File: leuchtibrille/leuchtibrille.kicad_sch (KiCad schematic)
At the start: 27 parts, among them J1 Conn_01x06_Male, J2 Conn_01x02_Female, J3 USB_C_Receptacle_USB2.0, J4 USB_C_Receptacle_USB2.0, J5 USB_C_Receptacle_USB2.0, SW1 SW_Push, U1 MT3420C, U2 MT3420C, U3 ESP32-WROOM-32

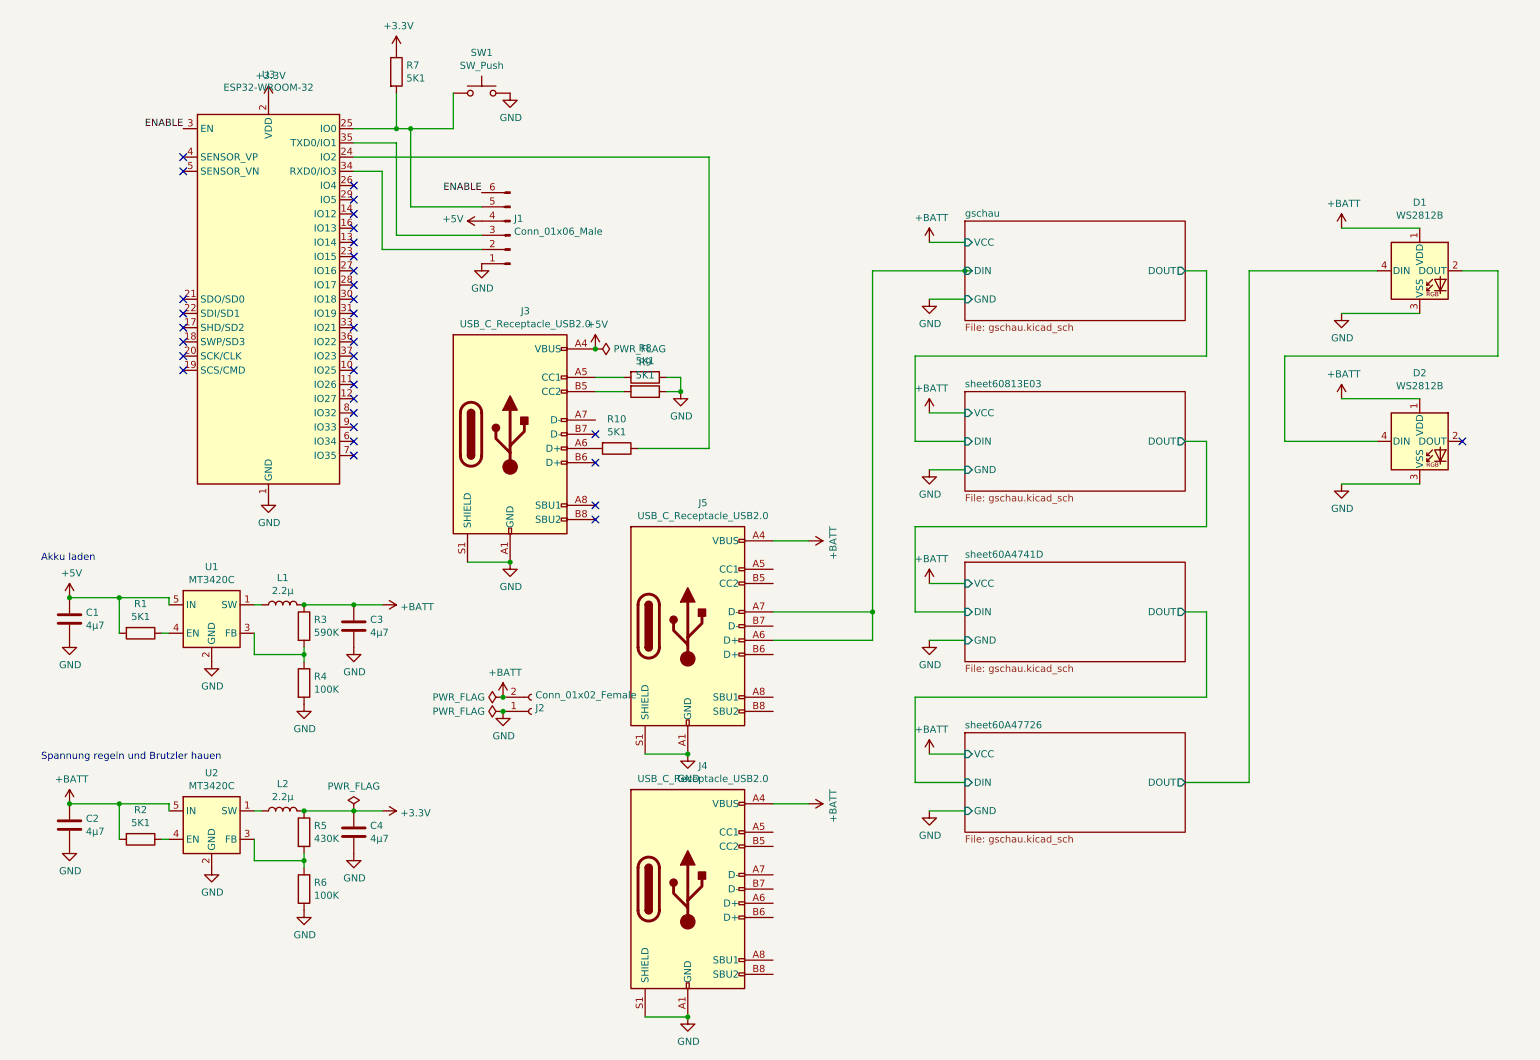
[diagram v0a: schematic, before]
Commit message: Upload of working version
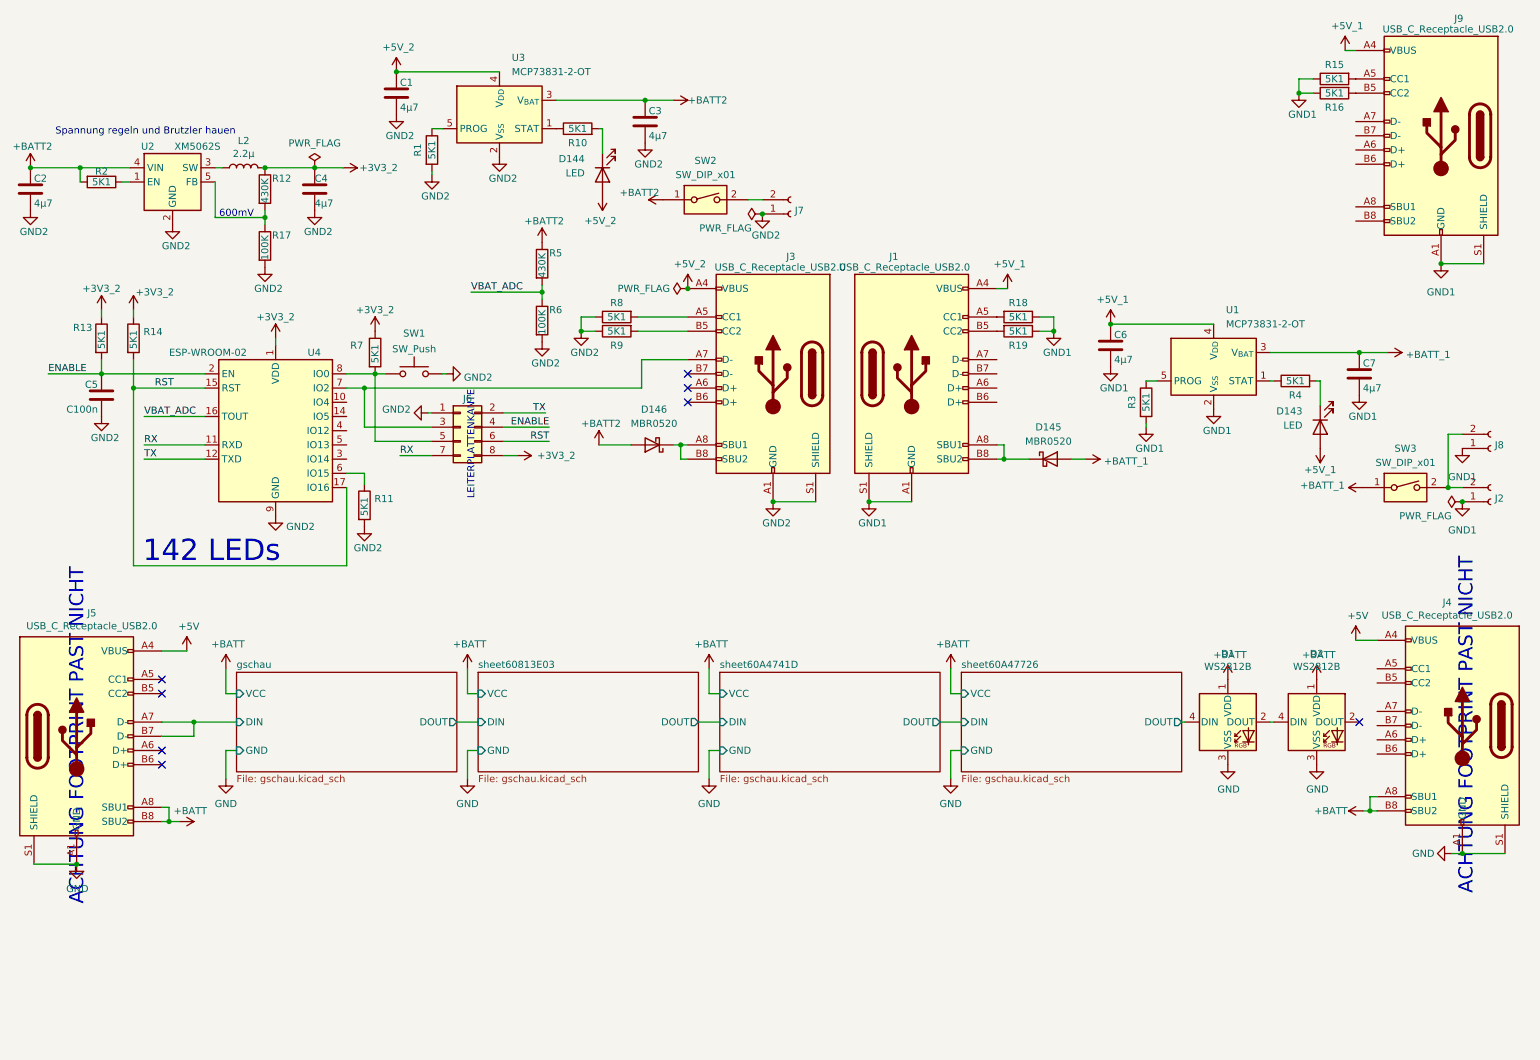
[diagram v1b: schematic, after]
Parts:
- removed J1: Conn_01x06_Male, Connector_PinHeader_2.54mm:PinHeader_1x06_P2.54mm_Vertical, symbol Connector:Conn_01x06_Male
- removed L1: 2.2µ, Inductor_SMD:L_1210_3225Metric_Pad1.42x2.65mm_HandSolder, symbol Device:L
- removed U1, U2: MT3420C, Package_TO_SOT_SMD:SOT-23-6, symbol Regulator_Switching:MT3608
- removed U3: ESP32-WROOM-32, RF_Module:ESP32-WROOM-32, symbol RF_Module:ESP32-WROOM-32
- added C5: C100n, Capacitor_SMD:C_0603_1608Metric_Pad1.08x0.95mm_HandSolder, symbol Device:C
- added C6, C7: 4µ7, Capacitor_SMD:C_1206_3216Metric, symbol Device:C
- added D143, D144: LED, LED_SMD:LED_0603_1608Metric, symbol Device:LED
- added D145, D146: MBR0520, Diode_SMD:D_SOD-123, symbol Diode:MBR0520
- added J1, J9: USB_C_Receptacle_USB2.0, Connector_USB:USB_C_Receptacle_HRO_TYPE-C-31-M-12, symbol Connector:USB_C_Receptacle_USB2.0
- added J6: Conn_02x04_Odd_Even, Connector_PinSocket_2.54mm:PinSocket_2x04_P2.54mm_Vertical, symbol Connector_Generic:Conn_02x04_Odd_Even
- added J7, J8: Conn_01x02_Female, Connector_JST:JST_PH_B2B-PH-K_1x02_P2.00mm_Vertical, symbol Connector:Conn_01x02_Female
- added R11, R13, R14, R15, R16, R18, R19: 5K1, Resistor_SMD:R_0603_1608Metric_Pad0.98x0.95mm_HandSolder, symbol Device:R
- added R12: 430K, Resistor_SMD:R_0603_1608Metric_Pad0.98x0.95mm_HandSolder, symbol Device:R
- added R17: 100K, Resistor_SMD:R_0603_1608Metric_Pad0.98x0.95mm_HandSolder, symbol Device:R
- added SW2, SW3: SW_DIP_x01, Button_Switch_SMD:SW_SPDT_PCM12, symbol Switch:SW_DIP_x01
- added U1, U3: MCP73831-2-OT, Package_TO_SOT_SMD:SOT-23-5, symbol Battery_Management:MCP73831-2-OT
- added U2: XM5062S, Package_TO_SOT_SMD:SOT-23-5, symbol Regulator_Switching:TLV62568DBV
- added U4: ESP-WROOM-02, RF_Module:ESP-WROOM-02, symbol RF_Module:ESP-WROOM-02
- J2: footprint Connector_PinSocket_2.54mm:PinSocket_1x02_P2.54mm_Vertical -> Connector_JST:JST_PH_B2B-PH-K_1x02_P2.00mm_Vertical
- J4, J5: footprint Eigene:USBC_THT -> TheBrutzlers_Lib:TYPEC-900L-ACP24; LCSC (none) -> C2982538
- R3: value 590K -> 5K1
- R4: value 100K -> 5K1
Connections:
- net +5V: now also J4.A4 (VBUS), J4.A9 (VBUS), J4.B4 (VBUS), J4.B9 (VBUS), J5.A4 (VBUS), J5.A9 (VBUS), J5.B4 (VBUS), J5.B9 (VBUS); no longer C1.1, J3.A4 (VBUS), J3.A9 (VBUS), J3.B4 (VBUS), J3.B9 (VBUS), R1.2
- net +BATT: now also J4.A8 (SBU1), J4.B8 (SBU2), J5.A8 (SBU1), J5.B8 (SBU2); no longer C2.1, C3.1, J2.2 (Pin_2), J4.A4 (VBUS), J4.A9 (VBUS), J4.B4 (VBUS), J4.B9 (VBUS), J5.A4 (VBUS), J5.A9 (VBUS), J5.B4 (VBUS), J5.B9 (VBUS), R2.2, R3.1
- net ENABLE: now also C5.2, J6.4 (Pin_4), R13.2, U4.2 (EN)
- net GND: no longer C1.2, C2.2, C3.2, C4.2, J2.1 (Pin_1), J3.A1 (GND), J3.A12 (GND), J3.B1 (GND), J3.B12 (GND), J3.S1 (SHIELD), R4.2, R6.2, R8.1, R9.1, SW1.2
- net gschau/DIN: now also J5.B7 (D-); no longer J5.A6 (D+)
- net at R10.1: now also U3.1 (STAT)
- net at R7.2, SW1.1: now also J6.5 (Pin_5), U4.8 (IO0)
- net at L2.1: now also U2.3 (SW)
- net VBAT_ADC: now reaches R5.2, R6.1
- net VBAT_ADC: now also U4.16 (TOUT)
- net at R2.1: now also U2.1 (EN)
- net at R4.1: now also U1.1 (STAT); no longer R3.2
- net at R1.1: now also U3.5 (PROG)
- net at J3.A6 (D+): no longer R10.2
- net at J3.A7 (D-): now also J6.3 (Pin_3), U4.7 (IO2)
- net at J3.A8 (SBU1): now also J3.B8 (SBU2), D146.1 (K)
- net +3V3 renamed +3V3_2
- net +3V3_2: now also J6.8 (Pin_8), R12.1, R13.1, R14.1, U4.1 (VDD); no longer R5.1
- new net: R12.2, R17.1, U2.5 (FB)
- new net: J1.A5 (CC1), R18.2
- new net: D145.1 (K), J1.A8 (SBU1), J1.B8 (SBU2)
- new net: J1.B5 (CC2), R19.2
- new net: R3.1, U1.5 (PROG)
- new net: J2.2 (Pin_2), J8.2 (Pin_2), SW3.2
- new net: D144.1 (K), R10.2
- new net: J7.2 (Pin_2), SW2.2
- new net: J9.A5 (CC1), R15.2
- new net: J9.B5 (CC2), R16.2
- new net: D143.1 (K), R4.2
- new net: R11.1, U4.6 (IO15)
- new net +5V_1: C6.1, D143.2 (A), J1.A4 (VBUS), J1.A9 (VBUS), J1.B4 (VBUS), J1.B9 (VBUS), J9.A4 (VBUS), J9.A9 (VBUS), J9.B4 (VBUS), J9.B9 (VBUS), U1.4 (V_{DD})
- new net +5V_2: C1.1, D144.2 (A), J3.A4 (VBUS), J3.A9 (VBUS), J3.B4 (VBUS), J3.B9 (VBUS), U3.4 (V_{DD})
- new net +BATT2: C2.1, C3.1, D146.2 (A), R2.2, R5.1, SW2.1, U2.4 (VIN), U3.3 (V_{BAT})
- new net +BATT_1: C7.1, D145.2 (A), SW3.1, U1.3 (V_{BAT})
- new net GND1: C6.2, C7.2, J1.A1 (GND), J1.A12 (GND), J1.B1 (GND), J1.B12 (GND), J1.S1 (SHIELD), J2.1 (Pin_1), J8.1 (Pin_1), J9.A1 (GND), J9.A12 (GND), J9.B1 (GND), J9.B12 (GND), J9.S1 (SHIELD), R15.1, R16.1, R18.1, R19.1, R3.2, U1.2 (V_{SS})
- new net GND2: C1.2, C2.2, C3.2, C4.2, C5.1, J3.A1 (GND), J3.A12 (GND), J3.B1 (GND), J3.B12 (GND), J3.S1 (SHIELD), J6.1 (Pin_1), J7.1 (Pin_1), R1.2, R11.2, R17.2, R6.2, R8.1, R9.1, SW1.2, U2.2 (GND), U3.2 (V_{SS}), U4.13 (GND), U4.18 (GND), U4.19 (GND), U4.9 (GND)
- new net RST: J6.6 (Pin_6), R14.2, U4.15 (RST), U4.17 (IO16)
- new net RX: J6.7 (Pin_7), U4.11 (RXD)
- new net TX: J6.2 (Pin_2), U4.12 (TXD)
- no-connect marks 33 -> 8
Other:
- note added: "142 LEDs"
- note added: "600mV"
- note added: "ACHTUNG FOOTPRINT PAST NICHT"
- note added: "LEITERPLATTENKANTE"
- note removed: "Akku laden"
- moved on the sheet: C1, C2, C3, C4, D1, D2, J3, J4, J5, L2, R1, R2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
